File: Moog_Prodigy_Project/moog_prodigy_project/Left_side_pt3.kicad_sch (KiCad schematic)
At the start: 54 parts, among them SW7 SW_Slide_DPDT, U12B MCP6562, U13 NE5532, U14 AD8001AR, U14C BF244A, U14E 4007, U2 NE5532, U2B2 OPA134

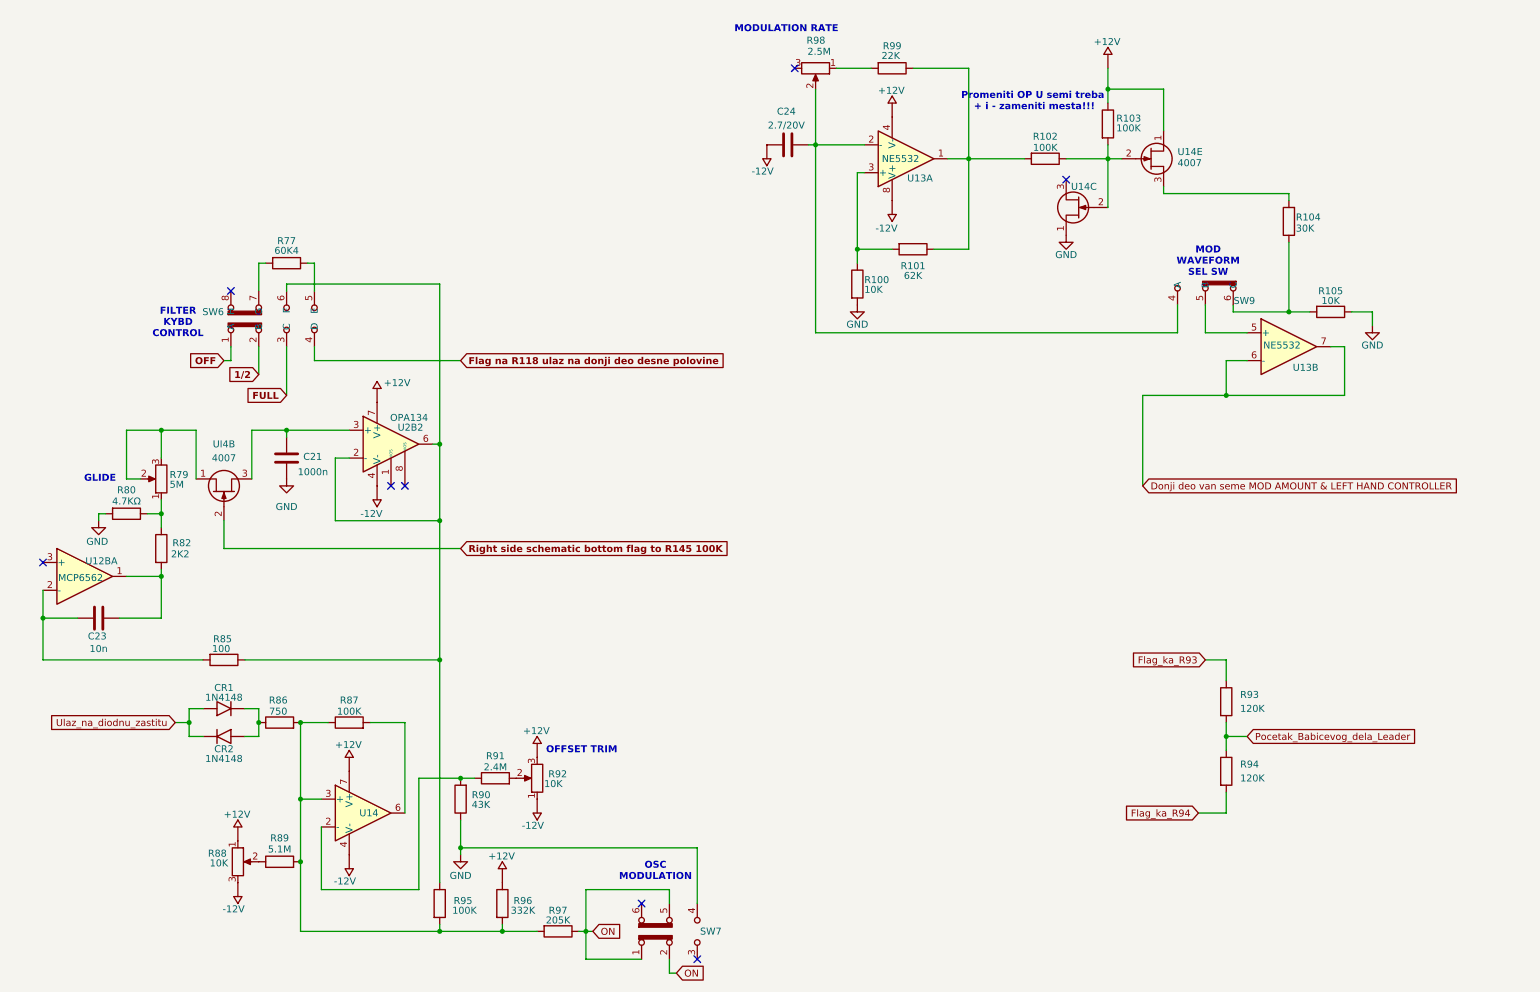
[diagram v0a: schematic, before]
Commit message: LM393BIPWR izmena, dodavanje spoljnih delova pt.2, 12.04.2026
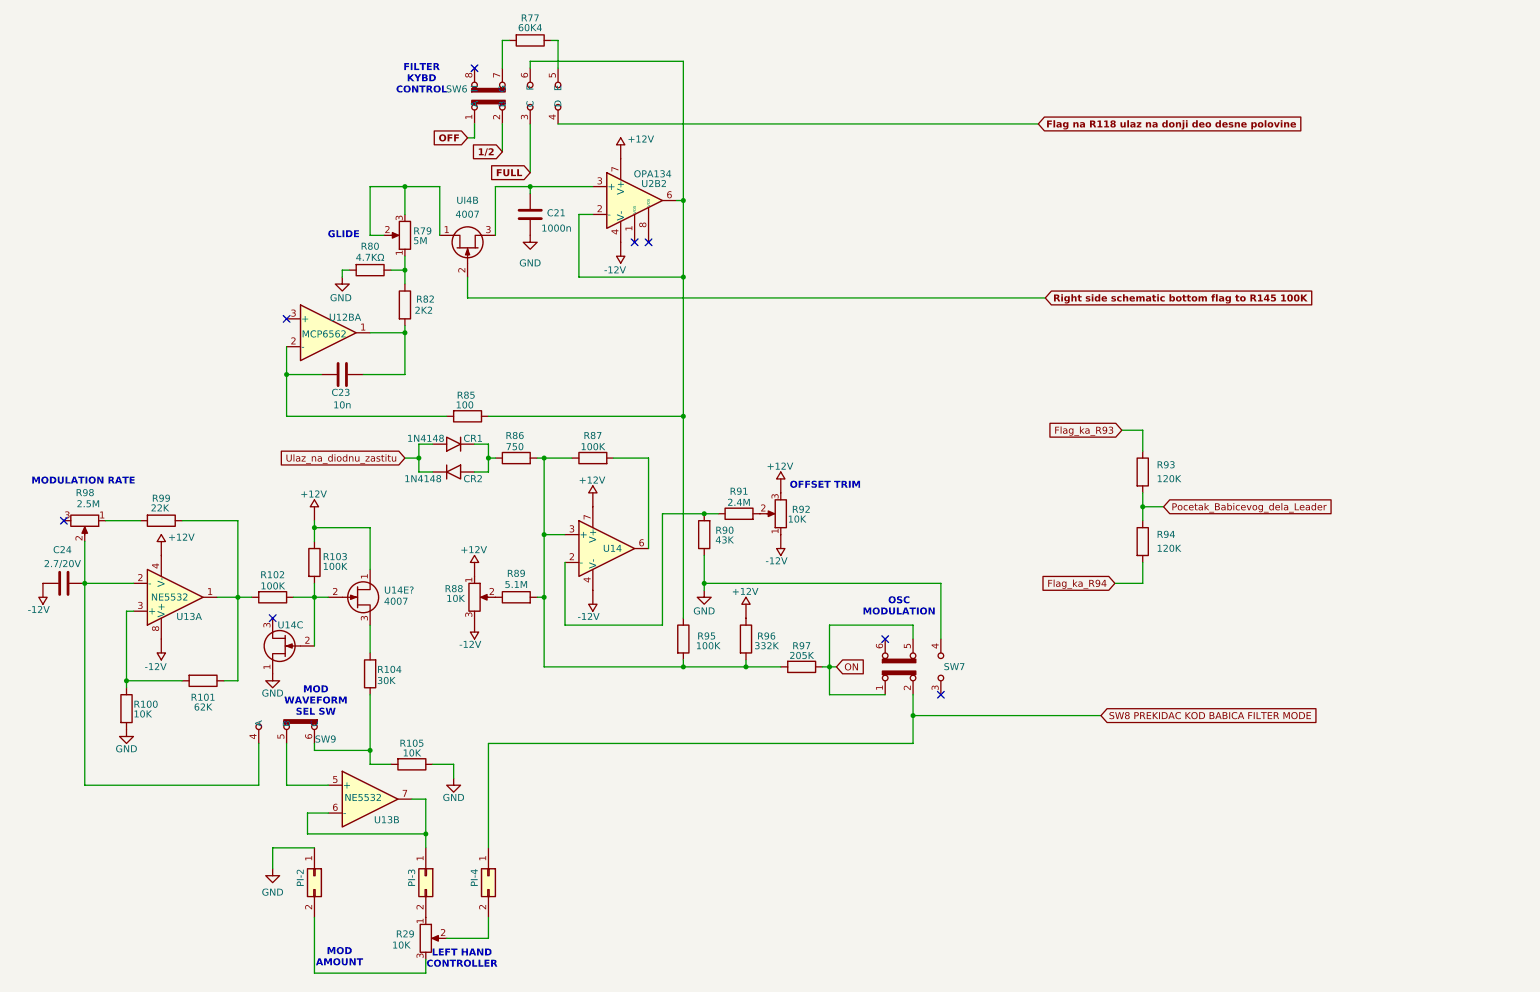
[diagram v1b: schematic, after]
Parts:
- added PI-2, PI-3, PI-4: Conn_02x01, symbol Connector_Generic:Conn_02x01
- added R29: 10K, symbol Device:R_Potentiometer
- renumbered U14E to U14E?
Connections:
- net GND: now also PI-2.1 (Pin_1)
- net ON: no longer SW7.2 (B)
- net Donji deo van seme MOD AMOUNT & LEFT HAND CONTROLLER: no longer names the net of U13.6 (-), U13.7
- net Donji deo van seme MOD AMOUNT & LEFT HAND CONTROLLER: now also PI-3.1 (Pin_1)
- new net: PI-3.2 (Pin_2), R29.1
- new net: PI-2.2 (Pin_2), R29.3
- new net: PI-4.2 (Pin_2), R29.2
- new net SW8 PREKIDAC KOD BABICA FILTER MODE: PI-4.1 (Pin_1), SW7.2 (B)
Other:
- note added: "LEFT HAND CONTROLLER"
- note added: "MOD AMOUNT"
- note removed: "Promeniti OP U semi treba + i - zameniti mesta!!!"
- moved on the sheet: C21, C23, C24, CR1, CR2, R100, R101, R102, R103, R104, R105, R77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
